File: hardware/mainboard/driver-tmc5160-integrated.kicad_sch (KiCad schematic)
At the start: 35 parts, among them M6 Micro-Fit 3.0, U1 TMC5160A-TA

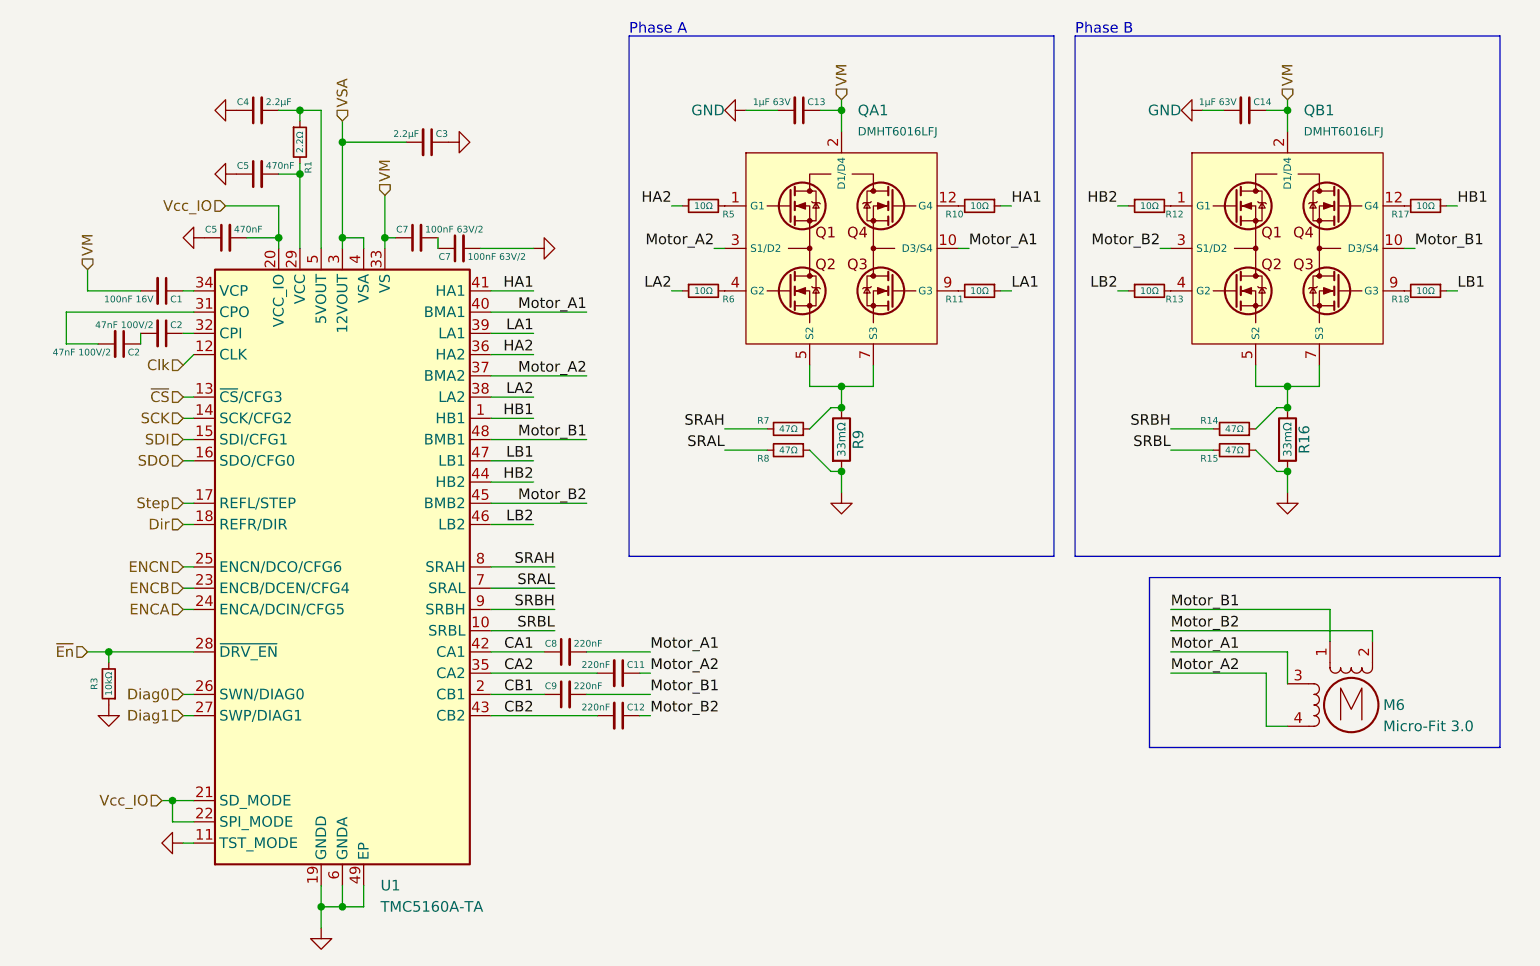
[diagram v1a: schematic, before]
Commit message: redoing board for version alpha 0.2
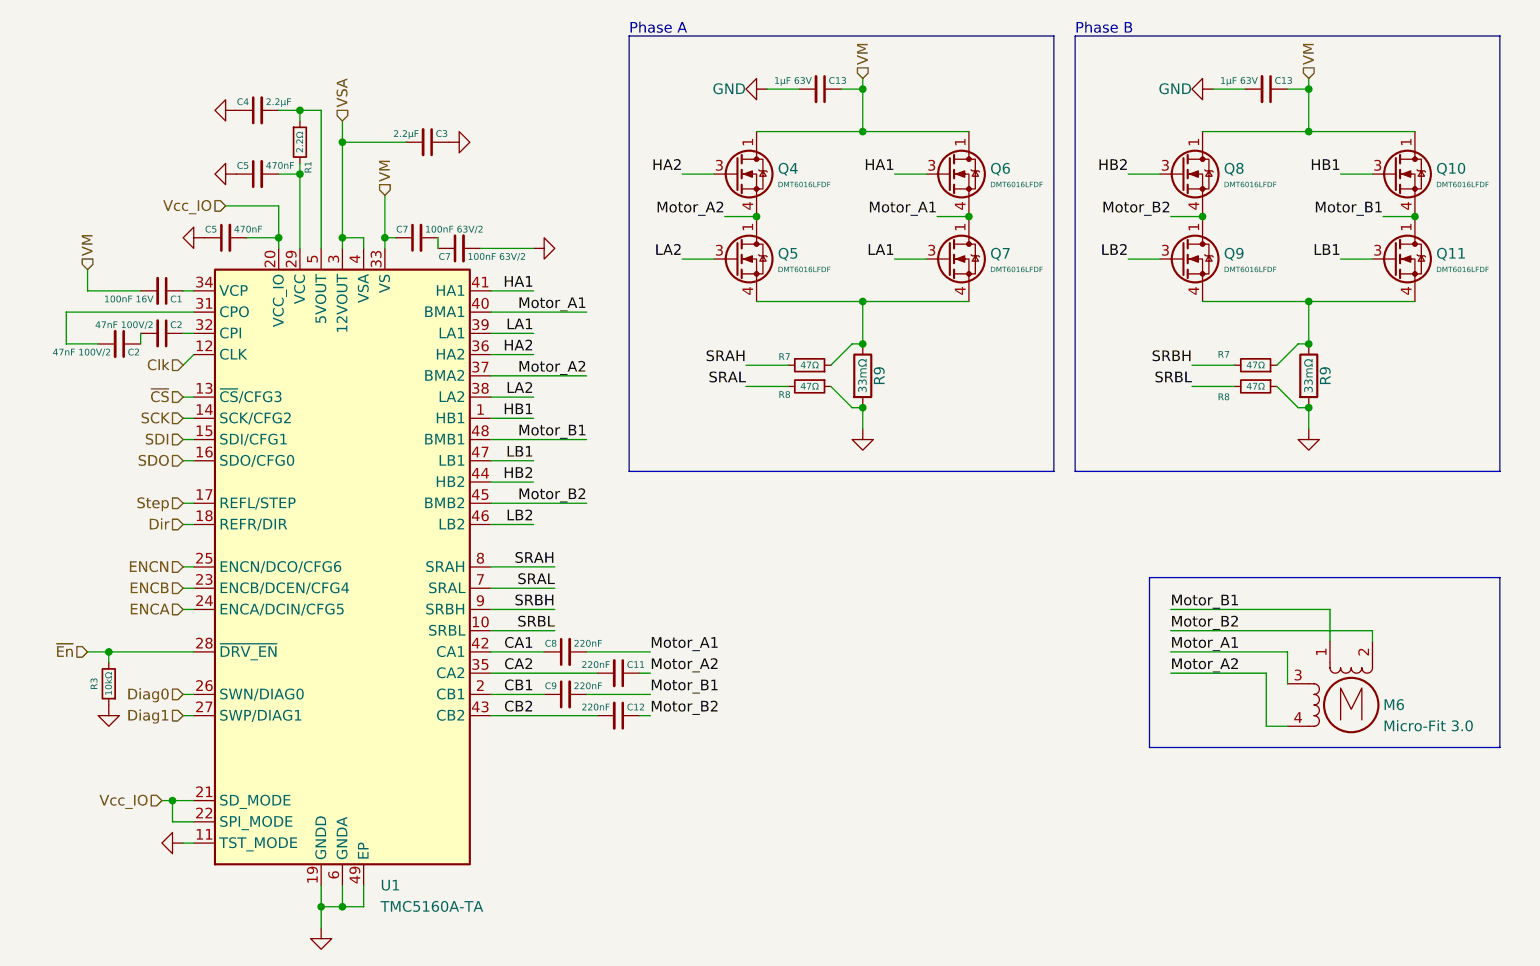
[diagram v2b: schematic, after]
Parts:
- removed C14: 1μF 63V, Capacitor_SMD:C_1206_3216Metric, symbol Device:C_Small
- removed QA1, QB1: DMHT6016LFJ, corevus:V-DFN5045-12-Type-B, symbol tmc5160-driver:DMHT6016LFJ
- removed R10, R11, R12, R13, R17, R18, R5, R6: 10Ω, AlphaLib:0402R, symbol Device:R_Small
- removed R14, R15: 47Ω, AlphaLib:0402R, symbol Device:R_Small
- removed R16: 33mΩ, Resistor_SMD:R_1206_3216Metric, symbol Device:R
- added C13: 1μF 63V, Capacitor_SMD:C_1206_3216Metric, symbol Device:C_Small
- added Q10, Q11, Q4, Q5, Q6, Q7, Q8, Q9: DMT6016LFDF, corevus:DMT6016LFDF, symbol corevus:DMT6016LFDF-7
- added R7, R8: 47Ω, AlphaLib:0402R, symbol Device:R_Small
- added R9: 33mΩ, Resistor_SMD:R_1206_3216Metric, symbol Device:R
- M6: footprint Connector_Molex:Molex_Micro-Fit_3.0_43650-0400_1x04_P3.00mm_Horizontal -> corevus:XKB_X3025WRS-04C
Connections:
- net GND: now also C13.2, R8.1, R9.2
- net HA1: now also Q6.3 (G)
- net HA2: now also Q4.3 (G)
- net HB1: now also Q10.3 (G)
- net HB2: now also Q8.3 (G)
- net LA1: now also Q7.3 (G)
- net LA2: now also Q5.3 (G)
- net LB1: now also Q11.3 (G)
- net LB2: now also Q9.3 (G)
- net Motor_A1: now also Q6.4 (S), Q6.7 (S), Q7.1 (D), Q7.2 (D), Q7.5 (D), Q7.6 (D), Q7.8 (D)
- net Motor_A2: now also Q4.4 (S), Q4.7 (S), Q5.1 (D), Q5.2 (D), Q5.5 (D), Q5.6 (D), Q5.8 (D)
- net Motor_B1: now also Q10.4 (S), Q10.7 (S), Q11.1 (D), Q11.2 (D), Q11.5 (D), Q11.6 (D), Q11.8 (D)
- net Motor_B2: now also Q8.4 (S), Q8.7 (S), Q9.1 (D), Q9.2 (D), Q9.5 (D), Q9.6 (D), Q9.8 (D)
- net SRBH: now also R7.2
- net SRBL: now also R8.2
- net VM: now also C13.1, Q10.1 (D), Q10.2 (D), Q10.5 (D), Q10.6 (D), Q10.8 (D), Q4.1 (D), Q4.2 (D), Q4.5 (D), Q4.6 (D), Q4.8 (D), Q6.1 (D), Q6.2 (D), Q6.5 (D), Q6.6 (D), Q6.8 (D), Q8.1 (D), Q8.2 (D), Q8.5 (D), Q8.6 (D), Q8.8 (D)
- net at R7.1, R9.1: now also Q5.4 (S), Q5.7 (S), Q7.4 (S), Q7.7 (S)
- new net: Q11.4 (S), Q11.7 (S), Q9.4 (S), Q9.7 (S), R7.1, R9.1
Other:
- moved on the sheet: C13, R7, R8, R9
